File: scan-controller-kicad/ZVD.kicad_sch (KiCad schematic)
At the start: 4 parts, among them Q3 DMMT5401, Q4 DMG2305UX

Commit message: Adding missing components Mfnrs and footprints
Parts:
- Q3: LCSC C154733 -> C154733
- Q4: LCSC C2940629 -> C2940629
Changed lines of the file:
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@@
         )
         (path "/ab6dbce1-4ecf-44ae-8f33-5f07e4f43ca9/13a79e71-0548-4260-a23d-d56f2aa50ff3"
-          (reference "R33") (unit 1)
+          (reference "R5") (unit 1)
         )
       )
@@
       (effects (font (size 1.27 1.27)) hide)
     )
-    (property "LCSC" " C154733" (at 144.145 83.185 0)
+    (property "LCSC" "C154733" (at 144.145 83.185 0)
       (effects (font (size 1.27 1.27)) hide)
     )
@@
         )
         (path "/ab6dbce1-4ecf-44ae-8f33-5f07e4f43ca9/13a79e71-0548-4260-a23d-d56f2aa50ff3"
-          (reference "Q8") (unit 2)
+          (reference "Q3") (unit 2)
         )
       )
@@
       (effects (font (size 1.27 1.27)) hide)
     )
-    (property "LCSC" " C154733" (at 128.905 83.185 0)
+    (property "LCSC" "C154733" (at 128.905 83.185 0)
       (effects (font (size 1.27 1.27)) hide)
     )
@@
         )
         (path "/ab6dbce1-4ecf-44ae-8f33-5f07e4f43ca9/13a79e71-0548-4260-a23d-d56f2aa50ff3"
-          (reference "Q8") (unit 1)
+          (reference "Q3") (unit 1)
         )
       )
@@
         )
         (path "/ab6dbce1-4ecf-44ae-8f33-5f07e4f43ca9/13a79e71-0548-4260-a23d-d56f2aa50ff3"
-          (reference "#PWR010") (unit 1)
+          (reference "#PWR013") (unit 1)
         )
       )
@@
         )
         (path "/ab6dbce1-4ecf-44ae-8f33-5f07e4f43ca9/13a79e71-0548-4260-a23d-d56f2aa50ff3"
-          (reference "R34") (unit 1)
+          (reference "R6") (unit 1)
         )
       )
@@
       (effects (font (size 1.27 1.27)) hide)
     )
-    (property "LCSC" " C2940629" (at 136.525 79.375 0)
+    (property "LCSC" "C2940629" (at 136.525 79.375 0)
       (effects (font (size 1.27 1.27)) hide)
     )
@@
         )
         (path "/ab6dbce1-4ecf-44ae-8f33-5f07e4f43ca9/13a79e71-0548-4260-a23d-d56f2aa50ff3"
-          (reference "Q9") (unit 1)
+          (reference "Q4") (unit 1)
         )
       )
@@
         )
         (path "/ab6dbce1-4ecf-44ae-8f33-5f07e4f43ca9/13a79e71-0548-4260-a23d-d56f2aa50ff3"
-          (reference "#PWR011") (unit 1)
+          (reference "#PWR014") (unit 1)
         )
       )

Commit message: BOM progress
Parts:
- R11, R14: Inventory (none) -> B
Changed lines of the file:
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@@
+      (effects (font (size 1.27 1.27)) hide)
+    )
+    (property "Inventory" "B" (at 126.365 93.98 0)
       (effects (font (size 1.27 1.27)) hide)
     )
@@
     )
     (property "LCSC" "C154733" (at 144.145 83.185 0)
+      (effects (font (size 1.27 1.27)) hide)
+    )
+    (property "Inventory" "" (at 144.145 83.185 0)
       (effects (font (size 1.27 1.27)) hide)
     )
@@
     )
     (property "LCSC" "C154733" (at 128.905 83.185 0)
+      (effects (font (size 1.27 1.27)) hide)
+    )
+    (property "Inventory" "" (at 128.905 83.185 0)
       (effects (font (size 1.27 1.27)) hide)
     )
@@
       (effects (font (size 1.27 1.27)) hide)
     )
+    (property "Inventory" "B" (at 146.685 93.98 0)
+      (effects (font (size 1.27 1.27)) hide)
+    )
     (pin "1")
     (pin "2")
@@
       (effects (font (size 1.27 1.27)) hide)
     )
+    (property "Inventory" "" (at 136.525 79.375 0)
+      (effects (font (size 1.27 1.27)) hide)
+    )

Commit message: BOM complete!
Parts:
- Q3, Q4: Inventory (none) -> E
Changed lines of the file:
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@@
       (effects (font (size 1.27 1.27)) hide)
     )
-    (property "Inventory" "" (at 144.145 83.185 0)
+    (property "Inventory" "E" (at 144.145 83.185 0)
       (effects (font (size 1.27 1.27)) hide)
     )
@@
       (effects (font (size 1.27 1.27)) hide)
     )
-    (property "Inventory" "" (at 128.905 83.185 0)
+    (property "Inventory" "E" (at 128.905 83.185 0)
       (effects (font (size 1.27 1.27)) hide)
     )
@@
       (effects (font (size 1.27 1.27)) hide)
     )
-    (property "Inventory" "" (at 136.525 79.375 0)
+    (property "Inventory" "E" (at 136.525 79.375 0)
       (effects (font (size 1.27 1.27)) hide)
     )

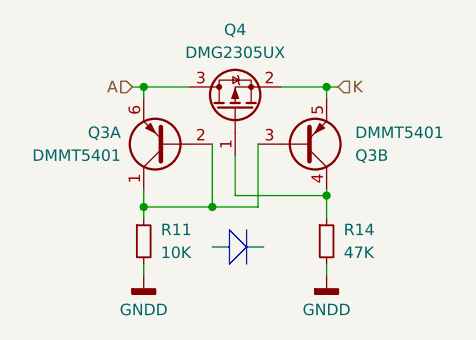
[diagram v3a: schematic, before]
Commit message: Starting PCB Layout
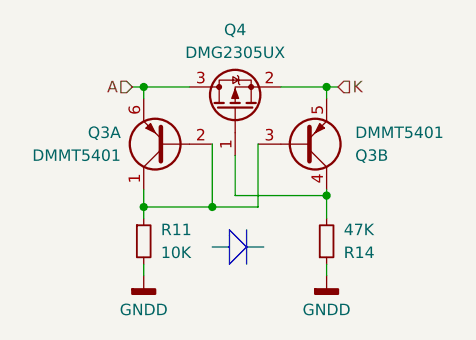
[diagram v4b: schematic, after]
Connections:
- net GNDD: now also R14.1; no longer R14.2
- net at Q3.4 (C2), Q4.1 (G): now also R14.2; no longer R14.1
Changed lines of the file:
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@@
     )
   )
-  (symbol (lib_id "Device:R_Small") (at 146.685 93.98 0) (unit 1)
-    (in_bom yes) (on_board yes) (dnp no) (fields_autoplaced)
-    (property "Reference" "R14" (at 148.59 92.71 0)
+  (symbol (lib_id "Device:R_Small") (at 146.685 93.98 0) (mirror x) (unit 1)
+    (in_bom yes) (on_board yes) (dnp no)
+    (property "Reference" "R14" (at 148.59 95.25 0)
       (effects (font (size 1.27 1.27)) (justify left))
     )
-    (property "Value" "47K" (at 148.59 95.25 0)
+    (property "Value" "47K" (at 148.59 92.71 0)
       (effects (font (size 1.27 1.27)) (justify left))
     )
